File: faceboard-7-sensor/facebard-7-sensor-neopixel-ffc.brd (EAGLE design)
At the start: 27 x 93.4 mm, 33 parts, among them J1 686114148922, J2 686114148922, Q1 QRE1113, Q2 QRE1113, Q3 QRE1113, Q4 QRE1113, Q5 QRE1113, Q6 QRE1113, Q7 QRE1113, U1 CD4051BE

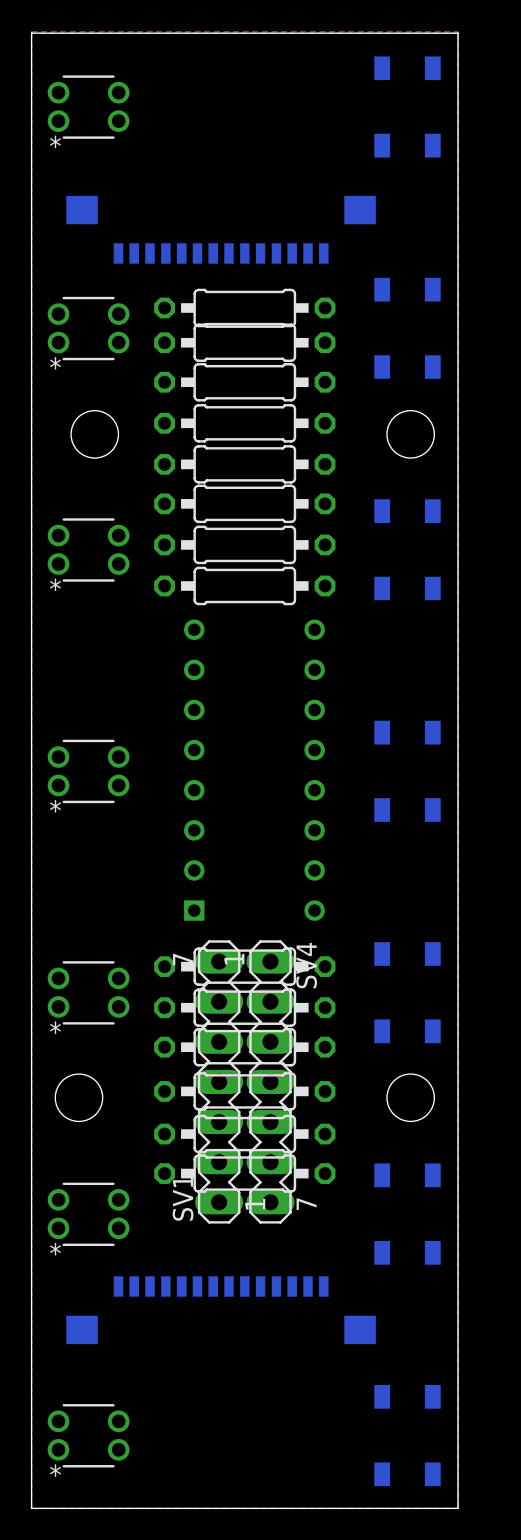
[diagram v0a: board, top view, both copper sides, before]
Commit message: add ffc
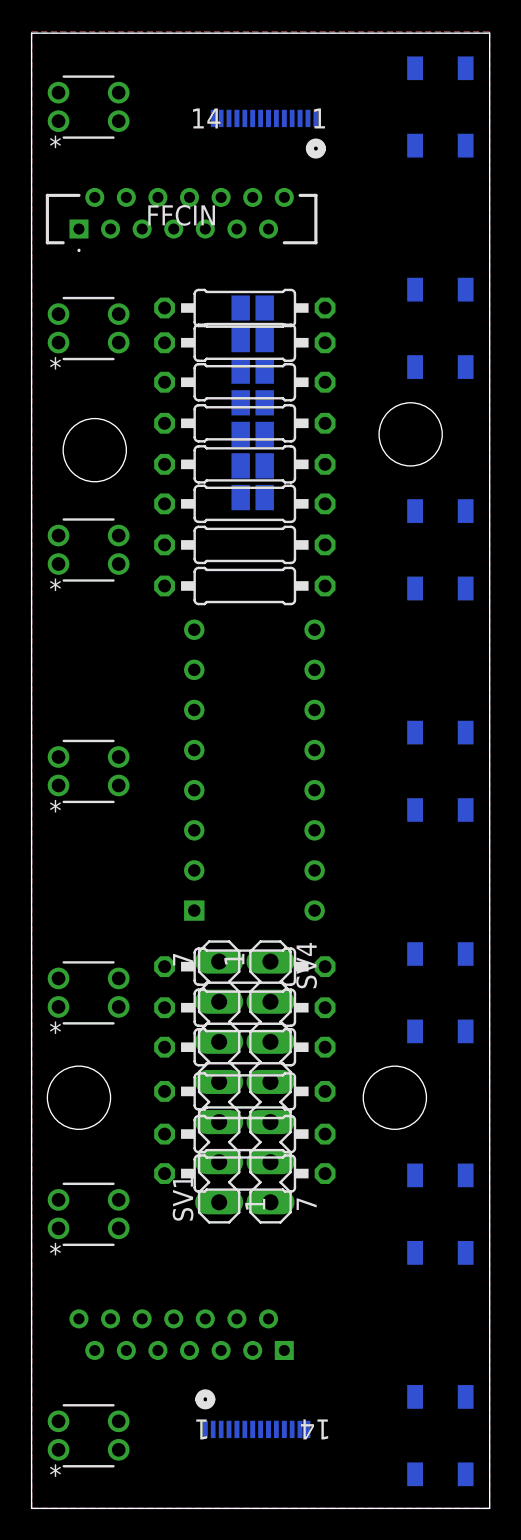
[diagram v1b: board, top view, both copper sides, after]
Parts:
- removed J2: 686114148922, 686114148922:686114148922
- added FFCIN, FFCOUT: 52806-1410, 52806-1410:528061410
- added J3: 1-1734592-4, 1-1734592-4:CONN_1-1734592-4_TYCO
- added SJ1, SJ2, SJ3, SJ4, SJ5, SJ6, SJ7: (no value), jumper:SJ
- J1: value 686114148922 -> 1-1734592-4; device 686114148922:686114148922 -> 1-1734592-4:CONN_1-1734592-4_TYCO
- moved J1 8.14 mm to (18.0, 86.0), turned to 0 degrees
- moved D1 2.08 mm to (25.9, 2.61)
- moved D2 2.08 mm to (25.9, 16.6)
- moved D3 2.08 mm to (25.9, 30.6)
- moved D4 2.08 mm to (25.9, 44.7)
- moved D5 2.08 mm to (25.9, 58.7)
- moved D6 2.08 mm to (25.9, 72.7)
- moved D7 2.08 mm to (25.9, 86.7)
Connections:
- net 3V: now also FFCIN.2, FFCOUT.13, J1.2, J3.13; no longer J1.13, J2.2
- net 5V: now also FFCIN.3, FFCOUT.12, J1.3, J3.12; no longer J1.12, J2.3
- net A: now also FFCIN.4, FFCOUT.11, J1.4, J3.11; no longer J1.11, J2.4
- net B: now also FFCIN.5, FFCOUT.10, J1.5, J3.10; no longer J1.10, J2.5
- net C: now also FFCIN.6, FFCOUT.9, J1.6, J3.9; no longer J1.9, J2.6
- net GND: now also FFCIN.1, FFCOUT.14, J1.1, J3.14; no longer J1.14, J1.MP1, J1.MP2, J2.1, J2.MP1, J2.MP2
- net LEDDIN: now also FFCIN.7, J1.7; no longer J2.7
- net LEDDOUT: now also FFCOUT.8, J3.8; no longer J1.8
- net N$18: no longer D3.4
- net SIG: now also SJ1.2, SJ2.2, SJ3.2, SJ4.2, SJ5.2, SJ6.2, SJ7.2
- net SIG1: now also FFCIN.8, FFCOUT.7, J1.14, J3.1, SJ1.1; no longer J1.1, J2.14
- net SIG2: now also FFCIN.9, FFCOUT.6, J1.13, J3.2, SJ2.1; no longer J1.2, J2.13
- net SIG3: now also FFCIN.10, FFCOUT.5, J1.12, J3.3, SJ3.1; no longer J1.3, J2.12
- net SIG4: now also FFCIN.11, FFCOUT.4, J1.11, J3.4, SJ4.1; no longer J1.4, J2.11
- net SIG5: now also FFCIN.12, FFCOUT.3, J1.10, J3.5, SJ5.1; no longer J1.5, J2.10
- net SIG6: now also FFCIN.13, FFCOUT.2, J1.9, J3.6, SJ6.1; no longer J1.6, J2.9
- net SIG7: now also FFCIN.14, FFCOUT.1, J1.8, J3.7, SJ7.1; no longer J1.7, J2.8
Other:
- board size 27 x 93.4 mm -> 29 x 93.4 mm
